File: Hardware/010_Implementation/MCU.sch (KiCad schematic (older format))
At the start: 17 parts, among them J1 2606-3356, J2 Conn_02x05_Odd_Even, SW1 SW_Push, U2 ESP32-DEVKITC-32D

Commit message: Board version 4.1
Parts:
- J1: symbol 2020-11-09_14-09-29:2606-3356 -> Board-rescue:2606-3356-2020-11-09_14-09-29
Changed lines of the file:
@@
 	4100 3350 5025 3350
 $Comp
-L 2020-11-09_14-09-29:2606-3356 J1
+L Board-rescue:2606-3356-2020-11-09_14-09-29 J1
 U 1 1 5FB5C146
 P 1325 6275
+AR Path="/5FB5C146" Ref="J1"  Part="1"
+AR Path="/5F52F099/5FB5C146" Ref="J1"  Part="1"
 F 0 "J1" H 1567 4888 60  0000 C CNN
 F 1 "2606-3356" H 1567 4994 60  0000 C CNN

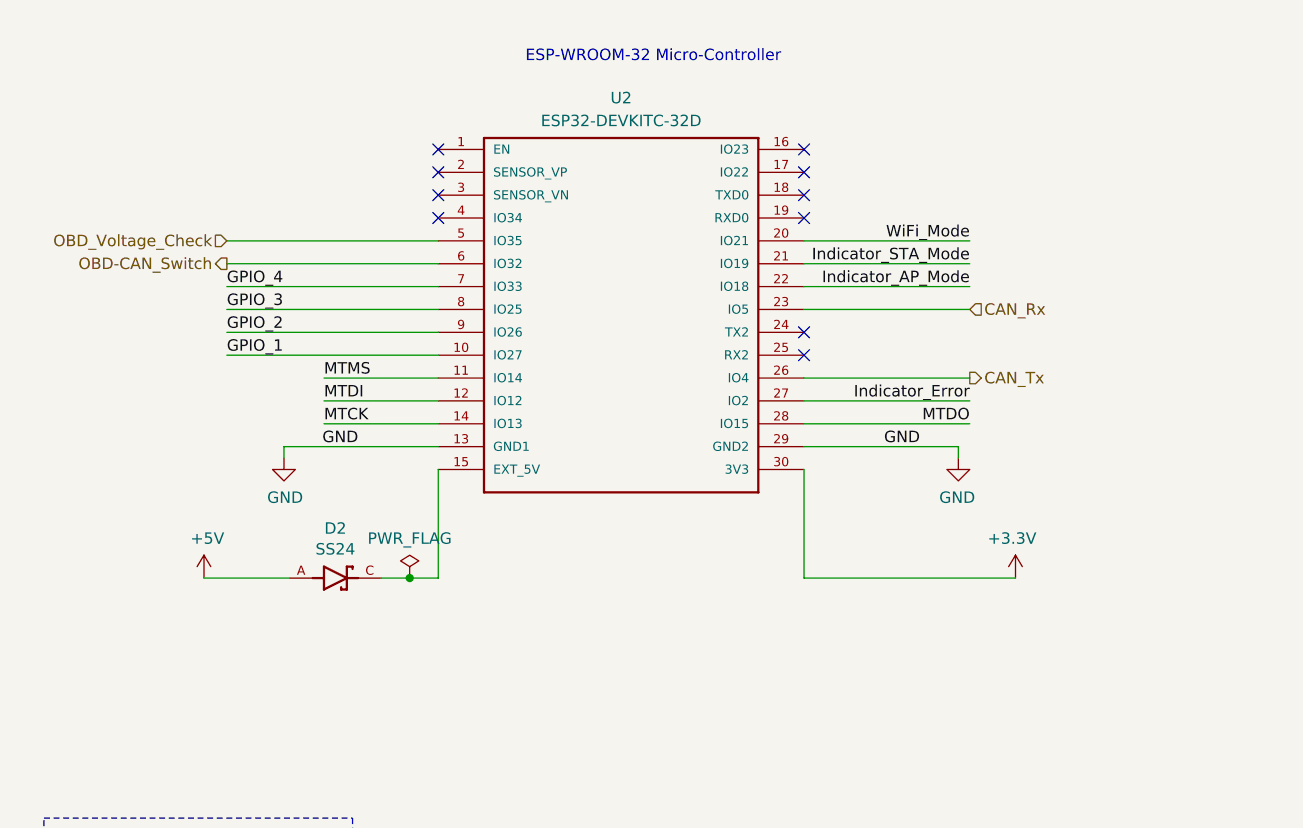
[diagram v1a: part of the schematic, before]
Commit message: Board Version 4.2
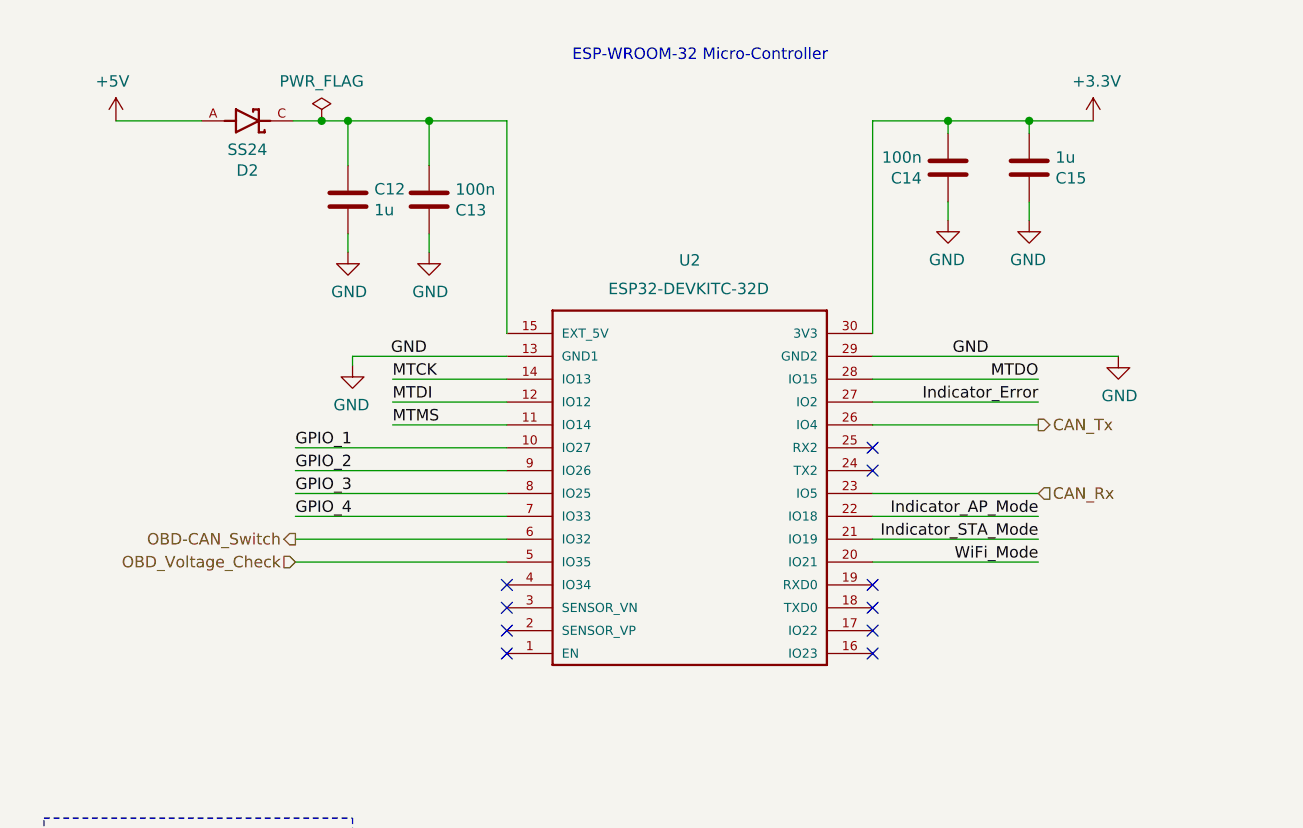
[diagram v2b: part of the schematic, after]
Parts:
- added C12, C15: 1u, symbol Device:C
- added C13, C14: 100n, symbol Device:C
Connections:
- net +3V3: now also C14.2, C15.2
- net GND: now also C12.2, C13.1, C14.1, C15.1
- net at D2.C, U2.15 (EXT_5V): now also C12.1, C13.2
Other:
- moved on the sheet: D2, U2
